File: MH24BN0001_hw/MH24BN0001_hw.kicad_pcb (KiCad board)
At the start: 2 copper layers, 7 parts, among them J1 ST-Link V2 Header, U1 STM32F401RBT6, U2 Accelerometer

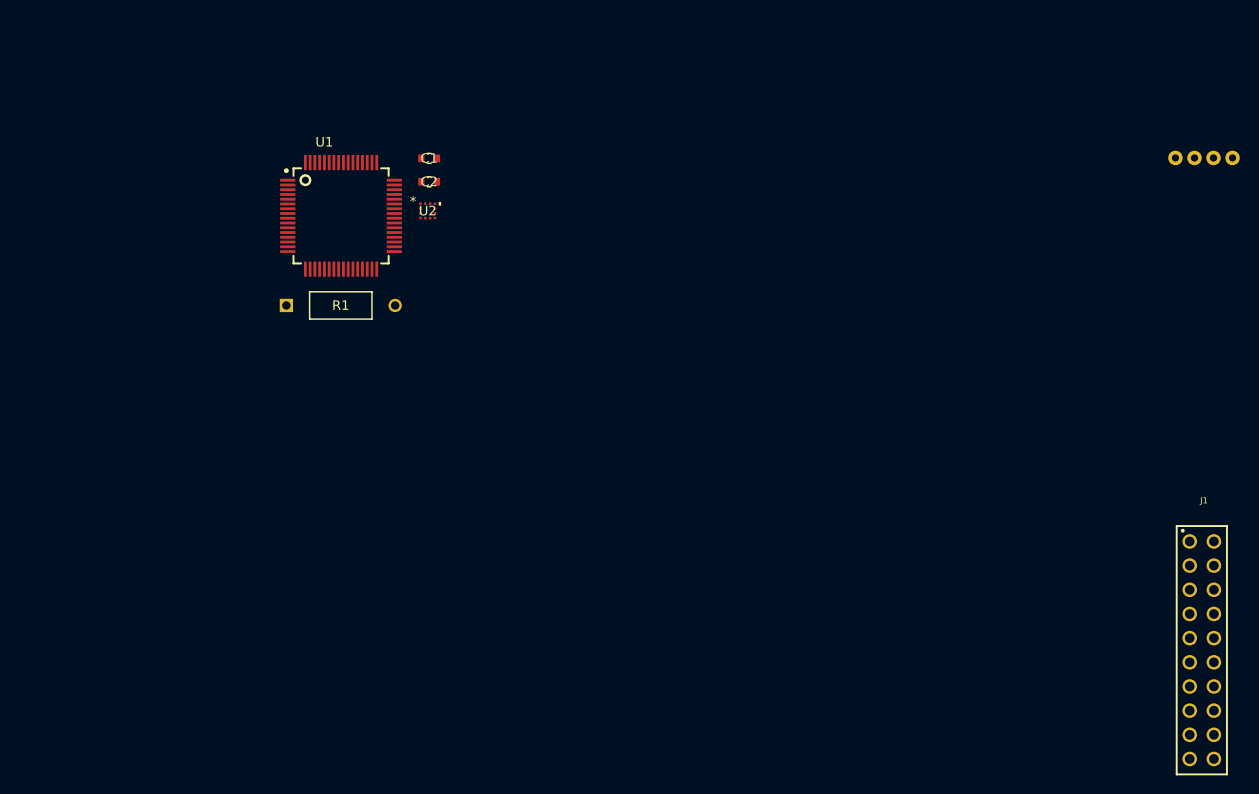
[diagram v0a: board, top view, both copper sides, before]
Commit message: starting PCB
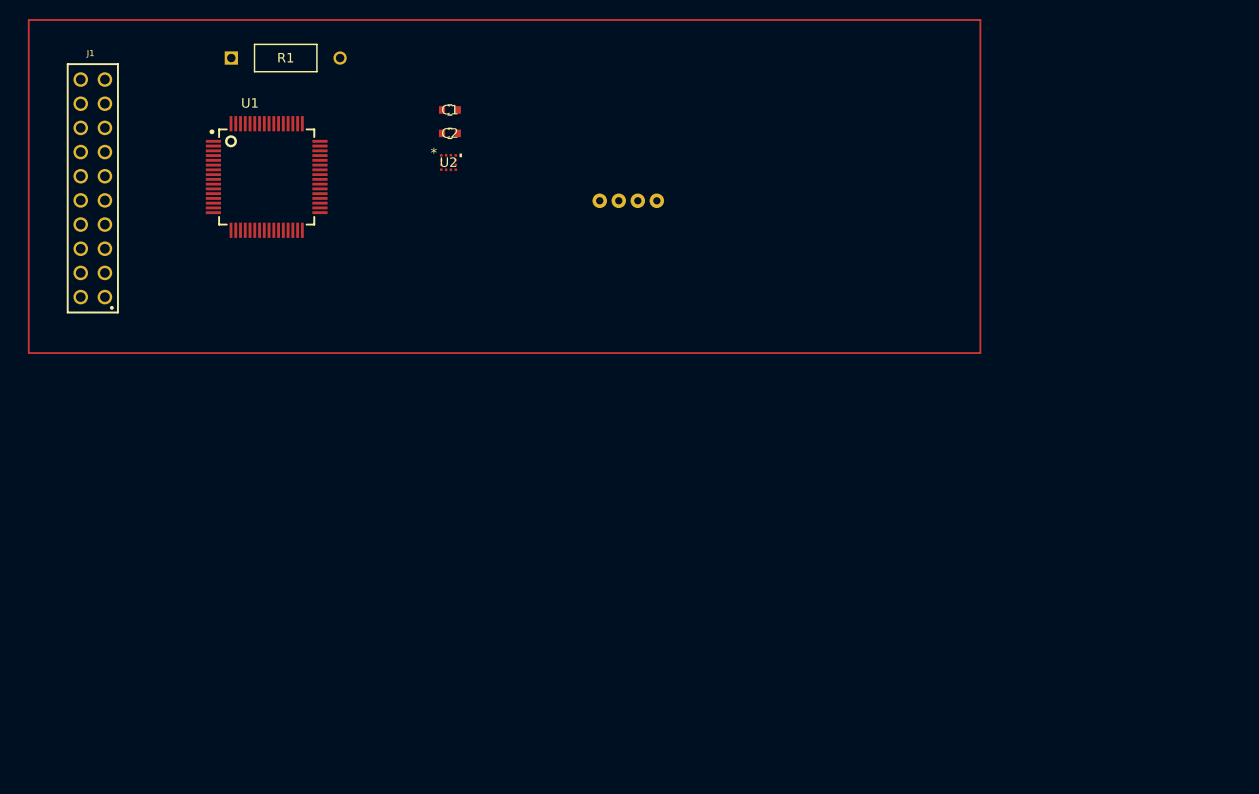
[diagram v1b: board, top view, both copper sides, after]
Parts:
- moved J1 126.2 mm to (33.2, 43.2), turned to 90 degrees
- moved SI1 60.7 mm to (89.5, 44.5)
- moved R1 26.6 mm to (47.8, 29.5)
- moved U1 8.82 mm to (51.5, 42.0)
- moved C1 5.54 mm to (70.8, 35.0)
- moved C2 5.54 mm to (70.8, 37.4)
- moved U2 5.54 mm to (70.6, 40.5)
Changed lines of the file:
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@@
 	(footprint "Library:QFP50P1200X1200X160-64N"
 		(layer "F.Cu")
-		(at 59.3163 46.0867)
+		(at 51.5 42)
 		(property "Reference" "U1"
 			(at -1.757345 -7.750405 0)
@@
 		)
 		(property "Value" "STM32F401RBT6"
-			(at 9.120105 7.672755 0)
+			(at 0 10 0)
 			(layer "F.Fab")
 			(effects
@@
 	(footprint "Library:61302021821"
 		(layer "F.Cu")
-		(at 149.77 91.73 -90)
+		(at 33.23 43.19 90)
 		(descr "<B>WR-PHD </B><BR> 2.54 mm Dual Socket Header,20 Pins")
 		(property "Reference" "J1"
-			(at -15.73 -0.23 180)
+			(at 14.19 -0.23 0)
 			(layer "F.SilkS")
 			(effects
@@
 		)
 		(property "Value" "ST-Link V2 Header"
-			(at -14.23 -0.23 180)
+			(at -14.23 -0.23 360)
 			(layer "F.Fab")
 			(effects
@@
 		)
 		(property "ROWS" "Dual"
-			(at 0 0 -90)
+			(at 0 0 90)
 			(unlocked yes)
 			(layer "F.Fab")
@@
 		)
 		(property "GENDER" "Socket Header"
-			(at 0 0 -90)
+			(at 0 0 90)
 			(unlocked yes)
 			(layer "F.Fab")
@@
 		)
 		(property "MOUNT" "THT"
-			(at 0 0 -90)
+			(at 0 0 90)
 			(unlocked yes)
 			(layer "F.Fab")
@@
 		)
 		(property "IR" "3A"
-			(at 0 0 -90)
+			(at 0 0 90)
 			(unlocked yes)
 			(layer "F.Fab")
@@
 		)
 		(property "VALUE" "61302021821"
-			(at 0 0 -90)
+			(at 0 0 90)
 			(unlocked yes)
 			(layer "F.Fab")
@@
 		)
 		(property "PACKAGING" "Tray"
-			(at 0 0 -90)
+			(at 0 0 90)
 			(unlocked yes)
 			(layer "F.Fab")
@@
 		)
 		(property "PART-NUMBER" "61302021821"
-			(at 0 0 -90)
+			(at 0 0 90)
 			(unlocked yes)
 			(layer "F.Fab")
@@
 		)
 		(property "DATASHEET-URL" "https://www.we-online.com/redexpert/spec/61302021821?ae"
-			(at 0 0 -90)
+			(at 0 0 90)
 			(unlocked yes)
 			(layer "F.Fab")
@@
 		)
 		(property "PITCH" "2.54mm"
-			(at 0 0 -90)
+			(at 0 0 90)
 			(unlocked yes)
 			(layer "F.Fab")
@@
 		)
 		(property "PINS" "20"
-			(at 0 0 -90)
+			(at 0 0 90)
 			(unlocked yes)
 			(layer "F.Fab")
@@
 		)
 		(property "TYPE" "Straight"
-			(at 0 0 -90)
+			(at 0 0 90)
 			(unlocked yes)
 			(layer "F.Fab")
@@
 		(attr through_hole)
 		(fp_line
-			(start -13.05 2.64)
-			(end -13.05 -2.64)
+			(start 13.05 -2.64)
+			(end 13.05 2.64)
 			(stroke
 				(width 0.2)
@@
 		)
 		(fp_line
-			(start 13.05 2.64)
-			(end -13.05 2.64)
+			(start -13.05 -2.64)
+			(end 13.05 -2.64)
 			(stroke
 				(width 0.2)
@@
 		)
 		(fp_line
-			(start -13.05 -2.64)
-			(end 13.05 -2.64)
+			(start 13.05 2.64)
+			(end -13.05 2.64)
 			(stroke
 				(width 0.2)
@@
 		)
 		(fp_line
-			(start 13.05 -2.64)
-			(end 13.05 2.64)
+			(start -13.05 2.64)
+			(end -13.05 -2.64)
 			(stroke
 				(width 0.2)
@@
 		)
 		(fp_line
-			(start -12.95 2.54)
-			(end 12.95 2.54)
+			(start 12.95 -2.54)
+			(end -12.95 -2.54)
 			(stroke
 				(width 0.1)
@@
 		)
 		(fp_line
-			(start 12.95 2.54)
-			(end 12.95 -2.54)
+			(start -12.95 -2.54)
+			(end -12.95 2.54)
 			(stroke
 				(width 0.1)
@@
 		)
 		(fp_line
-			(start -12.95 -2.54)
-			(end -12.95 2.54)
+			(start 12.95 2.54)
+			(end 12.95 -2.54)
 			(stroke
 				(width 0.1)
@@
 		)
 		(fp_line
-			(start 12.95 -2.54)
-			(end -12.95 -2.54)
+			(start -12.95 2.54)
+			(end 12.95 2.54)
 			(stroke
 				(width 0.1)
@@
 		)
 		(pad "1" thru_hole circle
-			(at -11.43 1.27 270)
+			(at -11.43 1.27 90)
 			(size 1.53 1.53)
 			(drill 1.02)
@@
 		)
 		(pad "2" thru_hole circle
-			(at -11.43 -1.27 270)
+			(at -11.43 -1.27 90)
 			(size 1.53 1.53)
 			(drill 1.02)
@@
 		)
 		(pad "3" thru_hole circle
-			(at -8.89 1.27 270)
+			(at -8.89 1.27 90)
 			(size 1.53 1.53)
 			(drill 1.02)
@@
 		)
 		(pad "4" thru_hole circle
-			(at -8.89 -1.27 270)
+			(at -8.89 -1.27 90)
 			(size 1.53 1.53)
 			(drill 1.02)
@@
 		)
 		(pad "5" thru_hole circle
-			(at -6.35 1.27 270)
+			(at -6.35 1.27 90)
 			(size 1.53 1.53)
 			(drill 1.02)
@@
 		)
 		(pad "6" thru_hole circle
-			(at -6.35 -1.27 270)
+			(at -6.35 -1.27 90)
 			(size 1.53 1.53)
 			(drill 1.02)
@@
 		)
 		(pad "7" thru_hole circle
-			(at -3.81 1.27 270)
+			(at -3.81 1.27 90)
 			(size 1.53 1.53)
 			(drill 1.02)
@@
 		)
 		(pad "8" thru_hole circle
-			(at -3.81 -1.27 270)
+			(at -3.81 -1.27 90)
 			(size 1.53 1.53)
 			(drill 1.02)
@@
 		)
 		(pad "9" thru_hole circle
-			(at -1.27 1.27 270)
+			(at -1.27 1.27 90)
 			(size 1.53 1.53)
 			(drill 1.02)
@@
 		)
 		(pad "10" thru_hole circle
-			(at -1.27 -1.27 270)
+			(at -1.27 -1.27 90)
 			(size 1.53 1.53)
 			(drill 1.02)
@@
 		)
 		(pad "11" thru_hole circle
-			(at 1.27 1.27 270)
+			(at 1.27 1.27 90)
 			(size 1.53 1.53)
 			(drill 1.02)
@@
 		)
 		(pad "12" thru_hole circle
-			(at 1.27 -1.27 270)
+			(at 1.27 -1.27 90)
 			(size 1.53 1.53)
 			(drill 1.02)
@@
 		)
 		(pad "13" thru_hole circle
-			(at 3.81 1.27 270)
+			(at 3.81 1.27 90)
 			(size 1.53 1.53)
 			(drill 1.02)
@@
 		)
 		(pad "14" thru_hole circle
-			(at 3.81 -1.27 270)
+			(at 3.81 -1.27 90)
 			(size 1.53 1.53)
 			(drill 1.02)
@@
 		)
 		(pad "15" thru_hole circle
-			(at 6.35 1.27 270)
+			(at 6.35 1.27 90)
 			(size 1.53 1.53)
 			(drill 1.02)
@@
 		)
 		(pad "16" thru_hole circle
-			(at 6.35 -1.27 270)
+			(at 6.35 -1.27 90)
 			(size 1.53 1.53)
 			(drill 1.02)
@@
 		)
 		(pad "17" thru_hole circle
-			(at 8.89 1.27 270)
+			(at 8.89 1.27 90)
 			(size 1.53 1.53)
 			(drill 1.02)
@@
 		)
 		(pad "18" thru_hole circle
-			(at 8.89 -1.27 270)
+			(at 8.89 -1.27 90)
 			(size 1.53 1.53)
 			(drill 1.02)
@@
 		)
 		(pad "19" thru_hole circle
-			(at 11.43 1.27 270)
+			(at 11.43 1.27 90)
 			(size 1.53 1.53)
 			(drill 1.02)
@@
 		)
 		(pad "20" thru_hole circle
-			(at 11.43 -1.27 270)
+			(at 11.43 -1.27 90)
 			(size 1.53 1.53)
 			(drill 1.02)
@@
 	(footprint "Library:2.2µF_cap"
 		(layer "F.Cu")
-		(at 68.5771 42.5023)
+		(at 70.7608 37.4156)
 		(tags "CL10A225KO8NNNC ")
 		(property "Reference" "C2"
@@
 			(polygon
 				(pts
-					(xy 68.1279 42.1531) (xy 69.0263 42.1531) (xy 69.0263 42.8515) (xy 68.1279 42.8515)
+					(xy 70.3116 37.0664) (xy 71.21 37.0664) (xy 71.21 37.7648) (xy 70.3116 37.7648)
 				)
 			)
@@
 	(footprint "Library:10 kΩ"
 		(layer "F.Cu")
-		(at 53.57 55.5)
+		(at 47.785 29.5)
 		(tags "CF14JT10K0 ")
 		(property "Reference" "R1"
@@
 		)
 		(property "Footprint" "Library:10 kΩ"
-			(at 0 0 0)
+			(at 0 0 360)
 			(layer "F.Fab")
 			(hide yes)
@@
 		)
 		(property "Datasheet" "https://www.digikey.com/en/products/detail/stackpole-electronics-inc/CF14JT10K0/1741265"
-			(at 0 0 0)
+			(at 0 0 360)
 			(layer "F.Fab")
 			(hide yes)
@@
 		)
 		(property "Description" ""
-			(at 0 0 0)
+			(at 0 0 360)
 			(layer "F.Fab")
 			(hide yes)
@@
 	(footprint "Library:1µF_cap"
 		(layer "F.Cu")
-		(at 68.5771 40.0419)
+		(at 70.7608 34.9552)
 		(tags "CL10B105KP8NNNC ")
 		(property "Reference" "C1"
@@
 			(polygon
 				(pts
-					(xy 68.1279 39.6927) (xy 69.0263 39.6927) (xy 69.0263 40.3911) (xy 68.1279 40.3911)
+					(xy 70.3116 34.606) (xy 71.21 34.606) (xy 71.21 35.3044) (xy 70.3116 35.3044)
 				)
 			)
@@
 	(footprint "Library:serial_interface"
 		(layer "F.Cu")
-		(at 150 40)
+		(at 89.5 44.5)
 		(property "Reference" "SI1"
 			(at 0 -4 0)
@@
 	(footprint "Library:acc"
 		(layer "F.Cu")
-		(at 68.4248 45.5652)
+		(at 70.6085 40.4785)
 		(tags "LIS2DTW12TR ")
 		(property "Reference" "U2"
@@
 		)
 	)
+	(gr_rect
+		(start 26.5 25.5)
+		(end 126.5 60.5)
+		(stroke
+			(width 0.2)
+			(type default)
+		)
+		(fill none)
+		(layer "F.Cu")
+		(net 3)
+	)
 )

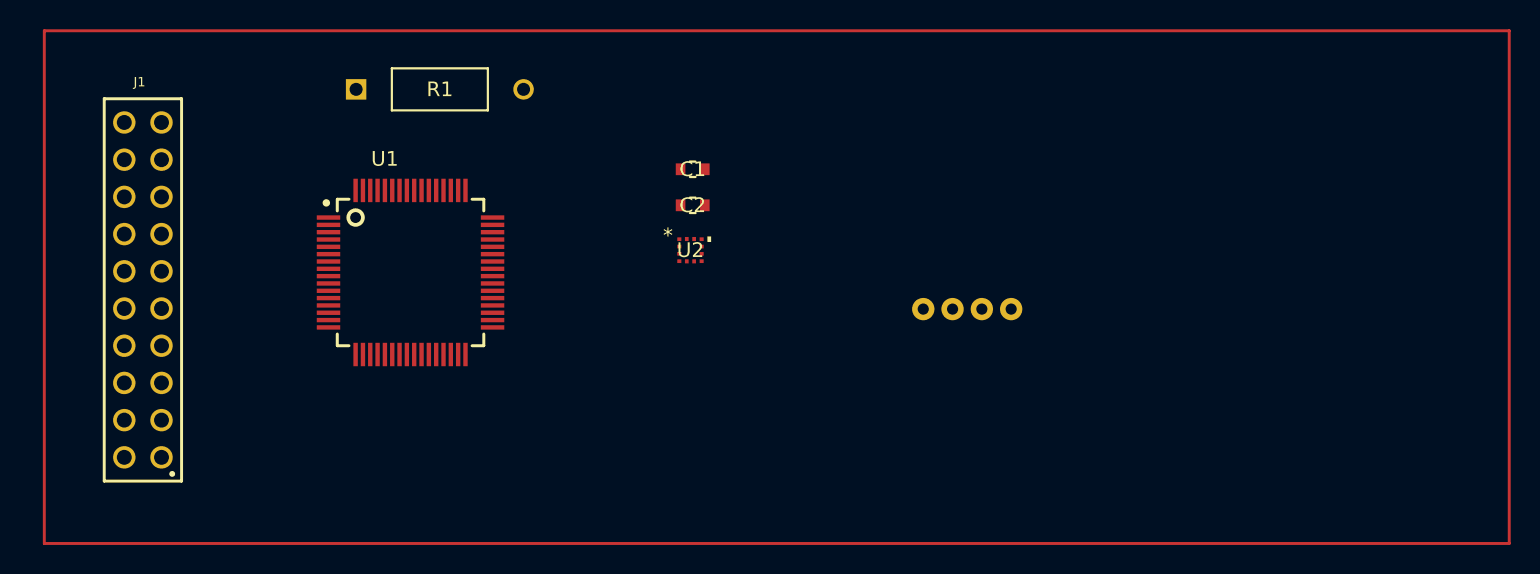
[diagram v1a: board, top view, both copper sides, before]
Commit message: finishing pcb, generating output files
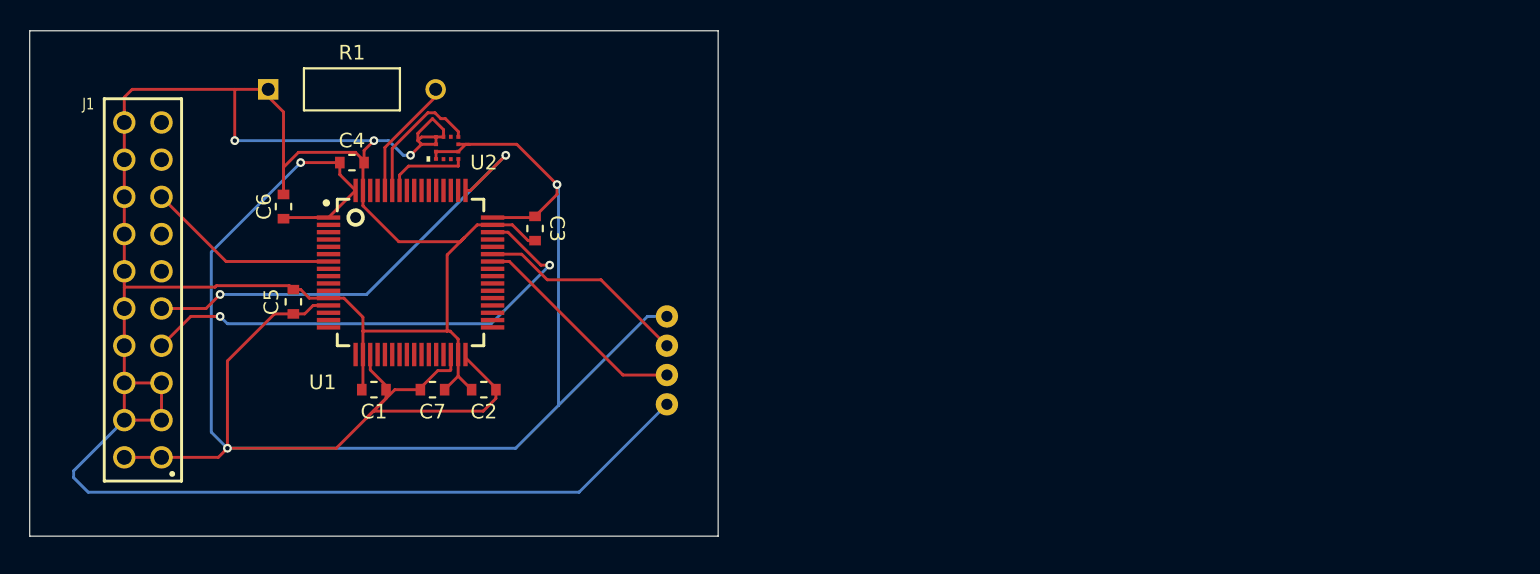
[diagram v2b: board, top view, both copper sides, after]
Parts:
- added C1: 1µF, Library:1µF_cap, F.Cu at (49.0, 50.0)
- added C2: 1µF, Library:1µF_cap, F.Cu at (56.5, 50.0)
- added C4: 1µF, Library:1µF_cap, F.Cu at (47.5, 34.5)
- added C5: 1µF, Library:1µF_cap, F.Cu at (43.5, 44.0)
- added C6: 1µF, Library:1µF_cap, F.Cu at (42.8, 37.5)
- moved C7 21.8 mm to (53.0, 50.0)
- moved SI1 20.8 mm to (69.0, 48.0), turned to -90 degrees
- moved U2 18.0 mm to (54.0, 33.5), turned to 180 degrees
- moved C3 11.5 mm to (60.0, 39.0), turned to -90 degrees
- moved R1 6.00 mm to (41.8, 29.5)
- renumbered C1 to C3, C2 to C7
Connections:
- C7 pad 1: Net-(U1-VCAP1) -> +3.3V
- U1 pad 30: Net-(U1-VCAP1) -> +3.3V
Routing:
- net GND: track 0.00 -> 188.7 mm, vias 0 -> 3
- net +3.3V: track 0.00 -> 156.9 mm, vias 0 -> 3
- net /SWDIO: track 0.00 -> 34.0 mm, vias 0 -> 2
- net /SWCLK: track 0.00 -> 31.6 mm, vias 0 -> 2
- net /MCU_TX: track 0.00 -> 15.1 mm
- net /MCU_RX: track 0.00 -> 14.5 mm
- net /NRST: track 0.00 -> 13.2 mm
- net /SDA: track 0.00 -> 9.29 mm
- net Net-(U1-BOOT0): track 0.00 -> 7.84 mm
- net /SCL: track 0.00 -> 5.80 mm
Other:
- board outline added: 47 x 34.5 mm
